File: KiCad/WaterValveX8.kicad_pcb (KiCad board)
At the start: 2 copper layers, 63.2 x 39.1 mm, 50 parts, among them J1 Conn_01x04_Male, J2 Barrel_Jack, J3 Conn_01x03_Male, J4 Conn_01x01_Male, J5 Conn_01x04_Male, J6 Screw_Terminal_01x03, J7 Screw_Terminal_01x03, J8 Screw_Terminal_01x03, J9 Screw_Terminal_01x02, Q1 IRLML2502, Q2 IRLML2502, Q3 IRLML2502, Q4 IRLML2502, U1 Project_DCDC_01, U2 SeedStudio XIAO ESP32 C3 v1, U3 L7805

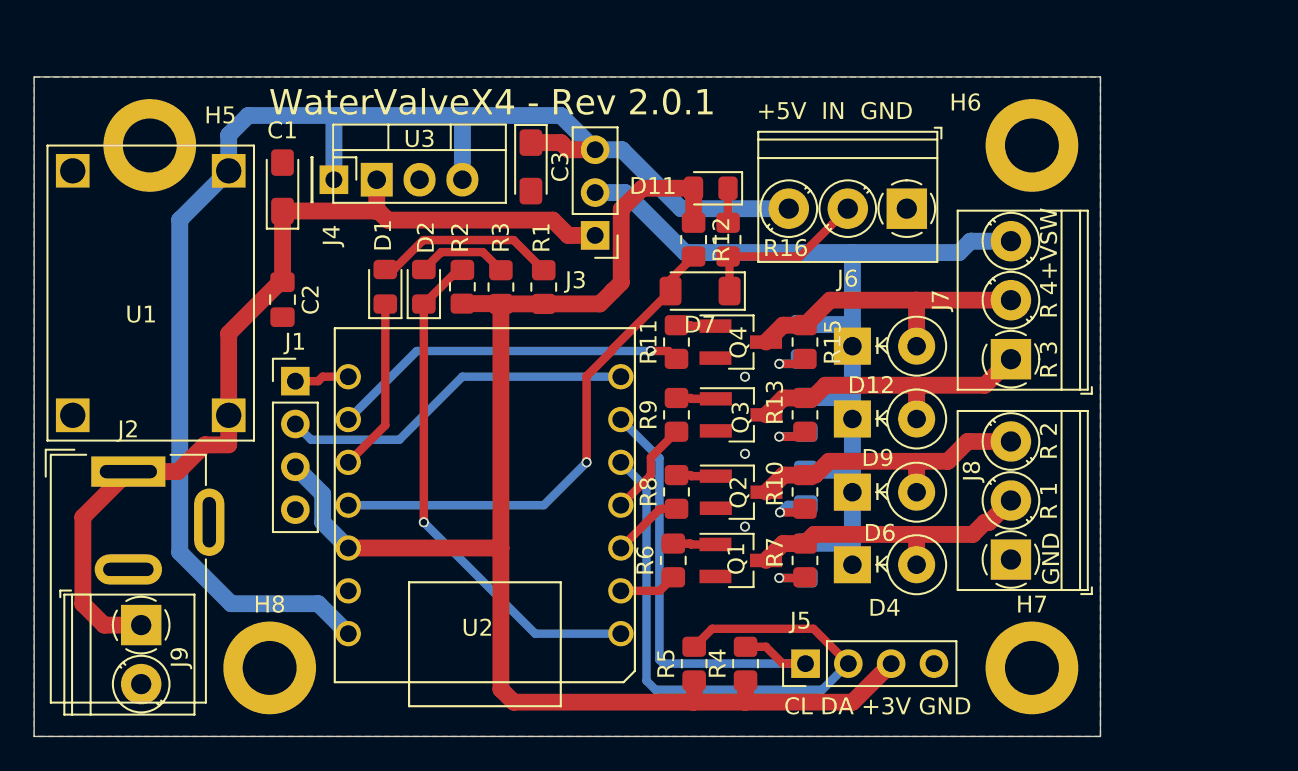
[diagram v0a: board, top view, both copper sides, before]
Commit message: First X8 layout
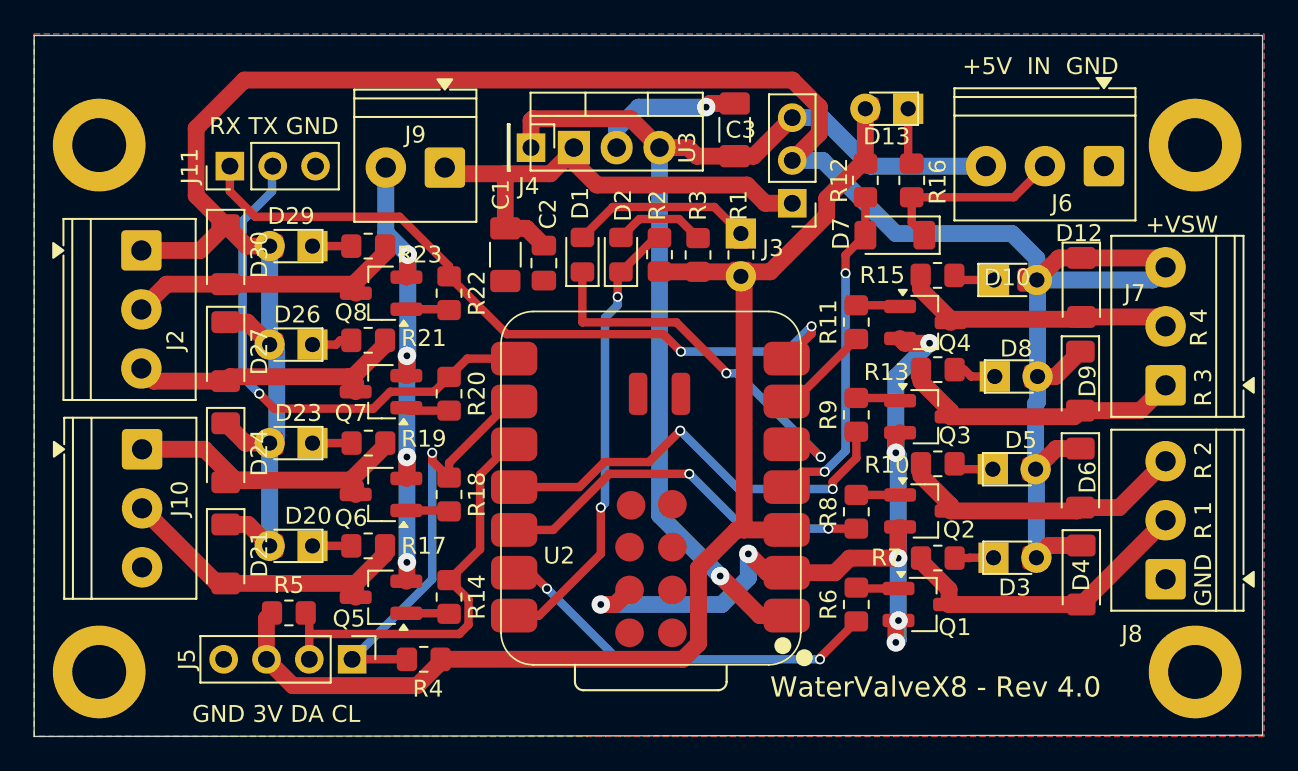
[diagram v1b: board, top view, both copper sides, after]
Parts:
- removed J1: Conn_01x04_Male, Connector_PinHeader_2.54mm:PinHeader_1x04_P2.54mm_Vertical
- removed U1: Project_DCDC_01, LOCAL1:DCDC_01
- added D13: LED, LED_SMD:LED_0805_2012Metric_Pad1.15x1.40mm_HandSolder, F.Cu at (186.5, 86.6)
- added D14: LED, LED_THT:LED_D3.0mm, B.Cu at (177.8, 94.0)
- added D15: LED, LED_THT:LED_D3.0mm, B.Cu at (192.8, 113.2)
- added D16: LED, LED_THT:LED_D3.0mm, B.Cu at (192.8, 108.0)
- added D17: LED, LED_THT:LED_D3.0mm, B.Cu at (192.9, 102.5)
- added D18: LED, LED_THT:LED_D3.0mm, B.Cu at (192.8, 96.8)
- added D19: LED, LED_THT:LED_D3.0mm, B.Cu at (152.4, 112.5)
- added D20: LED, LED_SMD:LED_0805_2012Metric_Pad1.15x1.40mm_HandSolder, F.Cu at (151.1, 112.5)
- added D21: 1N4148, Diode_SMD:D_MiniMELF, F.Cu at (147.2, 113.0)
- added D22: LED, LED_THT:LED_D3.0mm, B.Cu at (152.4, 106.4)
- added D23: LED, LED_SMD:LED_0805_2012Metric_Pad1.15x1.40mm_HandSolder, F.Cu at (151.1, 106.4)
- added D24: 1N4148, Diode_SMD:D_MiniMELF, F.Cu at (147.2, 107.0)
- added D25: LED, LED_THT:LED_D3.0mm, B.Cu at (152.4, 100.6)
- added D26: LED, LED_SMD:LED_0805_2012Metric_Pad1.15x1.40mm_HandSolder, F.Cu at (151.1, 100.6)
- added D27: 1N4148, Diode_SMD:D_MiniMELF, F.Cu at (147.2, 101.0)
- added D28: LED, LED_THT:LED_D3.0mm, B.Cu at (152.4, 94.7)
- added D29: LED, LED_SMD:LED_0805_2012Metric_Pad1.15x1.40mm_HandSolder, F.Cu at (151.1, 94.7)
- added D30: 1N4148, Diode_SMD:D_MiniMELF, F.Cu at (147.2, 95.2)
- added J10: Screw_Terminal_01x03, TerminalBlock_Phoenix:TerminalBlock_Phoenix_PT-1,5-3-3.5-H_1x03_P3.50mm_Horizontal, F.Cu at (142.3, 106.8)
- added J11: Conn_01x03_Pin, Connector_PinHeader_2.54mm:PinHeader_1x03_P2.54mm_Vertical, F.Cu at (147.5, 90.0)
- added Q5: IRLML2502, Package_TO_SOT_SMD:SOT-23_Handsoldering, F.Cu at (156.5, 115.6)
- added Q6: IRLML2502, Package_TO_SOT_SMD:SOT-23_Handsoldering, F.Cu at (156.5, 109.5)
- added Q7: IRLML2502, Package_TO_SOT_SMD:SOT-23_Handsoldering, F.Cu at (156.5, 103.4)
- added Q8: IRLML2502, Package_TO_SOT_SMD:SOT-23_Handsoldering, F.Cu at (156.5, 97.5)
- added R14: 1k, Resistor_SMD:R_0805_2012Metric_Pad1.20x1.40mm_HandSolder, F.Cu at (160.5, 115.6)
- added R17: 1k, Resistor_SMD:R_0805_2012Metric_Pad1.20x1.40mm_HandSolder, F.Cu at (155.7, 112.5)
- added R18: 1k, Resistor_SMD:R_0805_2012Metric_Pad1.20x1.40mm_HandSolder, F.Cu at (160.5, 109.5)
- added R19: 1k, Resistor_SMD:R_0805_2012Metric_Pad1.20x1.40mm_HandSolder, F.Cu at (155.7, 106.4)
- added R20: 1k, Resistor_SMD:R_0805_2012Metric_Pad1.20x1.40mm_HandSolder, F.Cu at (160.5, 103.5)
- added R21: 1k, Resistor_SMD:R_0805_2012Metric_Pad1.20x1.40mm_HandSolder, F.Cu at (155.7, 100.3)
- added R22: 1k, Resistor_SMD:R_0805_2012Metric_Pad1.20x1.40mm_HandSolder, F.Cu at (160.5, 97.5)
- added R23: 1k, Resistor_SMD:R_0805_2012Metric_Pad1.20x1.40mm_HandSolder, F.Cu at (155.7, 94.7)
- C1, C3: footprint Capacitor_Tantalum_SMD:CP_EIA-3216-18_Kemet-A_Pad1.58x1.35mm_HandSolder -> Capacitor_SMD:C_1206_3216Metric_Pad1.33x1.80mm_HandSolder
- D10, D3, D5, D8: moved to F.Cu
- D11: footprint LED_SMD:LED_0805_2012Metric_Pad1.15x1.40mm_HandSolder -> LED_THT:LED_D3.0mm; moved to B.Cu
- D12, D4, D6, D9: value 1N4007 -> 1N4148; footprint Diode_THT:D_DO-41_SOD81_P3.81mm_Vertical_KathodeUp -> Diode_SMD:D_MiniMELF
- J2: value Barrel_Jack -> Screw_Terminal_01x03; footprint LOCAL1:BarrelJack1 -> TerminalBlock_Phoenix:TerminalBlock_Phoenix_PT-1,5-3-3.5-H_1x03_P3.50mm_Horizontal
- U2: value SeedStudio XIAO ESP32 C3 v1 -> XIAO-ESP32-C6-SMD; footprint LOCAL1:XIAO_ESP32C3_THT -> LOCAL1:XIAO-ESP32-C6-SMD
- moved J9 32.6 mm to (160.2, 90.1), turned to 180 degrees
- moved J5 26.9 mm to (154.8, 119.2), turned to -90 degrees
- moved R5 24.2 mm to (151.0, 116.5), turned to 0 degrees
- moved R4 19.1 mm to (159.0, 119.2), turned to 180 degrees
- moved C2 15.7 mm to (166.1, 95.8)
- moved D12 14.0 mm to (198.0, 97.2), turned to -90 degrees
- moved C1 13.8 mm to (163.8, 95.2), turned to -90 degrees
- moved D9 13.7 mm to (197.9, 102.8), turned to -90 degrees
- moved D4 13.6 mm to (198.0, 114.2), turned to -90 degrees
- moved D6 13.5 mm to (197.9, 108.5), turned to -90 degrees
- moved J2 13.1 mm to (142.2, 95.0), turned to -90 degrees
- moved D10 12.8 mm to (193.8, 96.8), turned to 0 degrees
- moved D8 12.7 mm to (194.1, 102.5), turned to 0 degrees
- moved D11 12.6 mm to (187.7, 86.6)
- moved D5 12.4 mm to (194.0, 108.0), turned to 0 degrees
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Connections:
- D7 pad 2: /GPIO10 -> /D10
- J2 pad 1: /PwrIn -> +VSW
- J2 pad 2: GND -> /Relay8
- J2 pad 3: unconnected-(J2-Pad3) -> /Relay7
- R11 pad 1: /GPIO8 -> /D8
- R12 pad 2: /GPIO10 -> /D10
- R6 pad 1: /GPIO1 -> /D1
- R8 pad 1: /GPIO5 -> /D2
- R9 pad 1: /GPIO3 -> /D3
- U2 pad 1: /GPIO2 -> +5V
- U2 pad 10: Net-(D1-K) -> /SDA
- U2 pad 11: /GPIO10 -> /D3
- U2 pad 12: +3V3 -> /D2
- U2 pad 13: GND -> /D1
- U2 pad 14: +5V -> /GPIO2
- U2 pad 2: /GPIO1 -> GND
- U2 pad 3: /GPIO5 -> +3V3
- U2 pad 4: /GPIO3 -> /D10
- U2 pad 5: /SDA -> Net-(D1-K)
- U2 pad 6: /SCL -> /D8
- U2 pad 7: /TX -> /RX
- U2 pad 8: /RX -> /TX
- U2 pad 9: /GPIO8 -> /SCL
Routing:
- net +VSW: track 56.3 -> 148.1 mm
- net GND: track 0.00 -> 85.4 mm, vias 3 -> 12
- net /RX: track 3.25 -> 43.4 mm, vias 0 -> 2
- net /GPIO10: track 30.0 -> 0.00 mm, vias 1 -> 0
- net /PwrIn: track 55.8 -> 28.9 mm
- net /D3: track 0.00 -> 25.7 mm, vias 0 -> 2
- net /D1: track 0.00 -> 23.4 mm, vias 0 -> 2
- net /D2: track 0.00 -> 23.0 mm, vias 0 -> 2
- net +5V: track 85.6 -> 63.5 mm, vias 0 -> 1
- net /GPIO8: track 21.3 -> 0.00 mm, vias 1 -> 0
- net /D10: track 0.00 -> 19.9 mm, vias 0 -> 2
- net /Relay6: track 0.00 -> 19.2 mm
- net /Relay5: track 0.00 -> 18.3 mm
- net /Relay7: track 0.00 -> 16.9 mm
- net /Relay8: track 0.00 -> 16.8 mm
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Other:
- board size 63.2 x 39.1 mm -> 72.9 x 41.6 mm
- board text added: "(C) 2025 Hans Rune Bue <email@hansrune.net>"
- board text added: "GND 3V DA CL"
- board text added: "RX TX GND"
- board text added: "WaterValveX8 - Rev 4.0"
- board text removed: "(C) 2023 Hans Rune Bue <email@hansrune.net>"
- board text removed: "CL DA +3V GND"
- board text removed: "WaterValveX4 - Rev 2.0.1"
